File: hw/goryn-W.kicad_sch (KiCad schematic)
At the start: 19 parts, among them J1 Conn_FFC_30, U3 MT3520B, U4 MT3520B

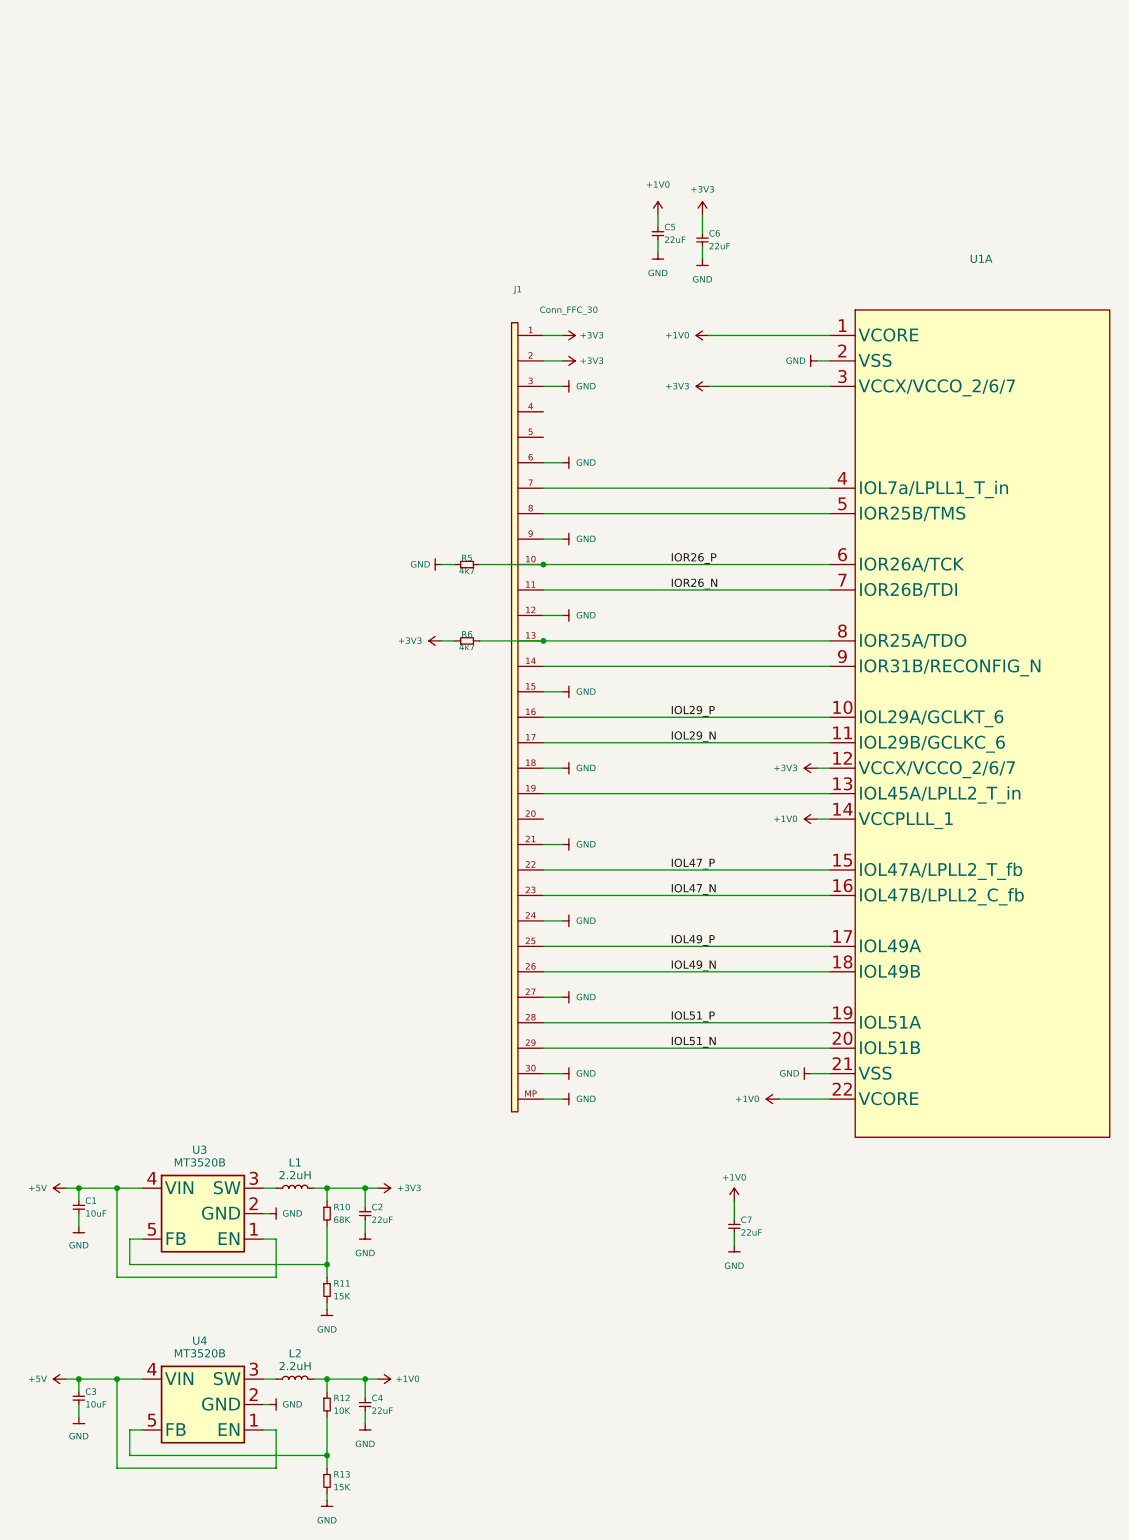
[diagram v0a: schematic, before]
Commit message: happy kicad 8
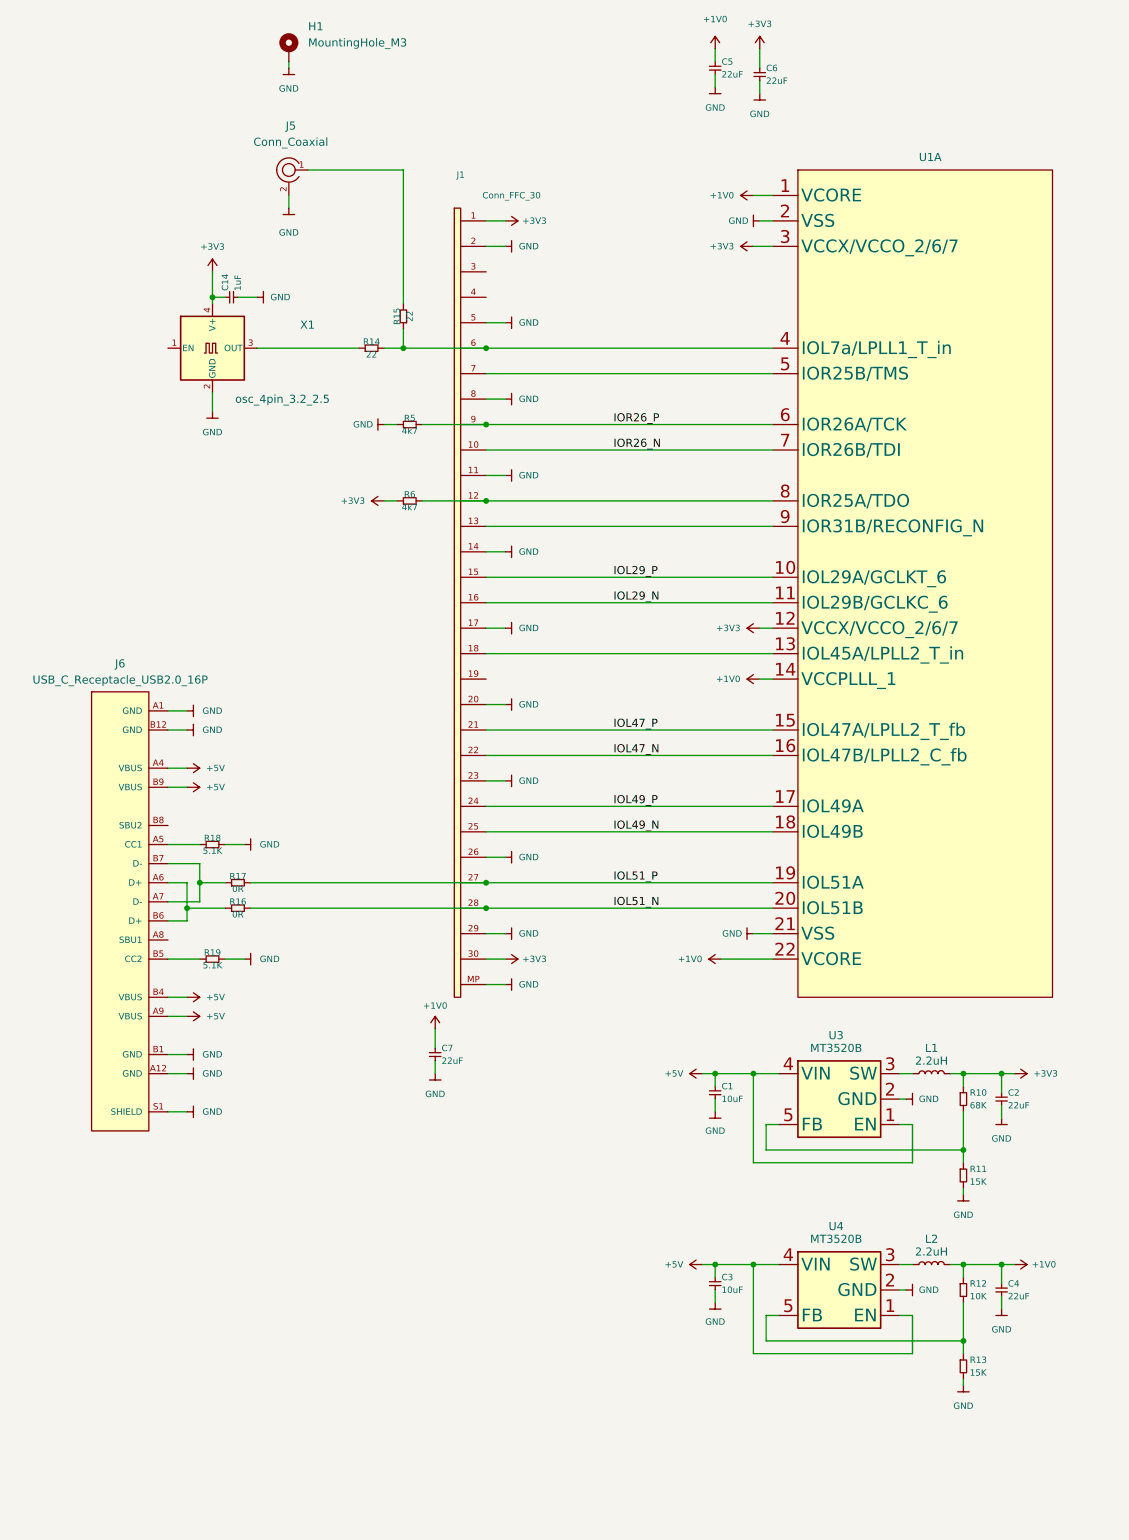
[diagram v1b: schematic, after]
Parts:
- added C14: 1uF, AI6YP:C_0603_1608Metric, symbol AI6YP:C
- added H1: MountingHole_M3, AI6YP:MountingHole_3.2mm_M3_Pad_Via, symbol AI6YP:MountingHole_M3
- added J5: Conn_Coaxial, AI6YP:U.FL_Hirose_U.FL-R-SMT-1_Vertical, symbol AI6YP:IPEX
- added J6: USB_C_Receptacle_USB2.0_16P, AI6YP:USB_C_Receptacle_GCT_USB4105-xx-A_16P_TopMnt_Horizontal, symbol AI6YP:USB_C_Receptacle_USB2.0_16P
- added R14, R15: 22, AI6YP:R_0603_1608Metric, symbol AI6YP:R
- added R16, R17: 0R, AI6YP:R_0603_1608Metric, symbol AI6YP:R
- added R18, R19: 5.1K, AI6YP:R_0603_1608Metric, symbol AI6YP:R
- added X1: osc_4pin_3.2_2.5, AI6YP:Crystal_SMD_EuroQuartz_MT-4Pin_3.2x2.5mm_HandSoldering, symbol AI6YP:osc_4pin_3.2_2.5
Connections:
- net +3V3: now also J1.30 (Pin_30), C14.1, X1.4 (V+); no longer J1.2 (Pin_2)
- net +5V: now also J6.A4 (VBUS), J6.A9 (VBUS), J6.B4 (VBUS), J6.B9 (VBUS)
- net GND: now also J1.11 (Pin_11), J1.14 (Pin_14), J1.17 (Pin_17), J1.2 (Pin_2), J1.20 (Pin_20), J1.23 (Pin_23), J1.26 (Pin_26), J1.29 (Pin_29), J1.5 (Pin_5), J1.8 (Pin_8), C14.2, H1.1, J5.2 (Ext), J6.A1 (GND), J6.A12 (GND), J6.B1 (GND), J6.B12 (GND), J6.S1 (SHIELD), R18.2, R19.2, X1.2 (GND); no longer J1.12 (Pin_12), J1.15 (Pin_15), J1.18 (Pin_18), J1.21 (Pin_21), J1.24 (Pin_24), J1.27 (Pin_27), J1.3 (Pin_3), J1.30 (Pin_30), J1.6 (Pin_6), J1.9 (Pin_9)
- net IOL29_N: now also J1.16 (Pin_16); no longer J1.17 (Pin_17)
- net IOL29_P: now also J1.15 (Pin_15); no longer J1.16 (Pin_16)
- net IOL47_N: now also J1.22 (Pin_22); no longer J1.23 (Pin_23)
- net IOL47_P: now also J1.21 (Pin_21); no longer J1.22 (Pin_22)
- net IOL49_N: now also J1.25 (Pin_25); no longer J1.26 (Pin_26)
- net IOL49_P: now also J1.24 (Pin_24); no longer J1.25 (Pin_25)
- net IOL51_N: now also J1.28 (Pin_28), R16.2; no longer J1.29 (Pin_29)
- net IOL51_P: now also J1.27 (Pin_27), R17.2; no longer J1.28 (Pin_28)
- net IOR26_N: now also J1.10 (Pin_10); no longer J1.11 (Pin_11)
- net IOR26_P: now also J1.9 (Pin_9); no longer J1.10 (Pin_10)
- net at R6.2, U1.8 (IOR25A/TDO): now also J1.12 (Pin_12); no longer J1.13 (Pin_13)
- net at U1.13 (IOL45A/LPLL2_T_in): now also J1.18 (Pin_18); no longer J1.19 (Pin_19)
- net at U1.4 (IOL7a/LPLL1_T_in): now also J1.6 (Pin_6), R14.2, R15.1; no longer J1.7 (Pin_7)
- net at U1.5 (IOR25B/TMS): now also J1.7 (Pin_7); no longer J1.8 (Pin_8)
- net at U1.9 (IOR31B/RECONFIG_N): now also J1.13 (Pin_13); no longer J1.14 (Pin_14)
- new net: J6.A7 (D-), J6.B7 (D-), R17.1
- new net: J5.1 (In), R15.2
- new net: J6.A5 (CC1), R18.1
- new net: R14.1, X1.3 (OUT)
- new net: J6.B5 (CC2), R19.1
- new net: J6.A6 (D+), J6.B6 (D+), R16.1
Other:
- moved on the sheet: C1, C2, C3, C4, C5, C6, C7, J1, L1, L2, R10, R11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

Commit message: finished routing
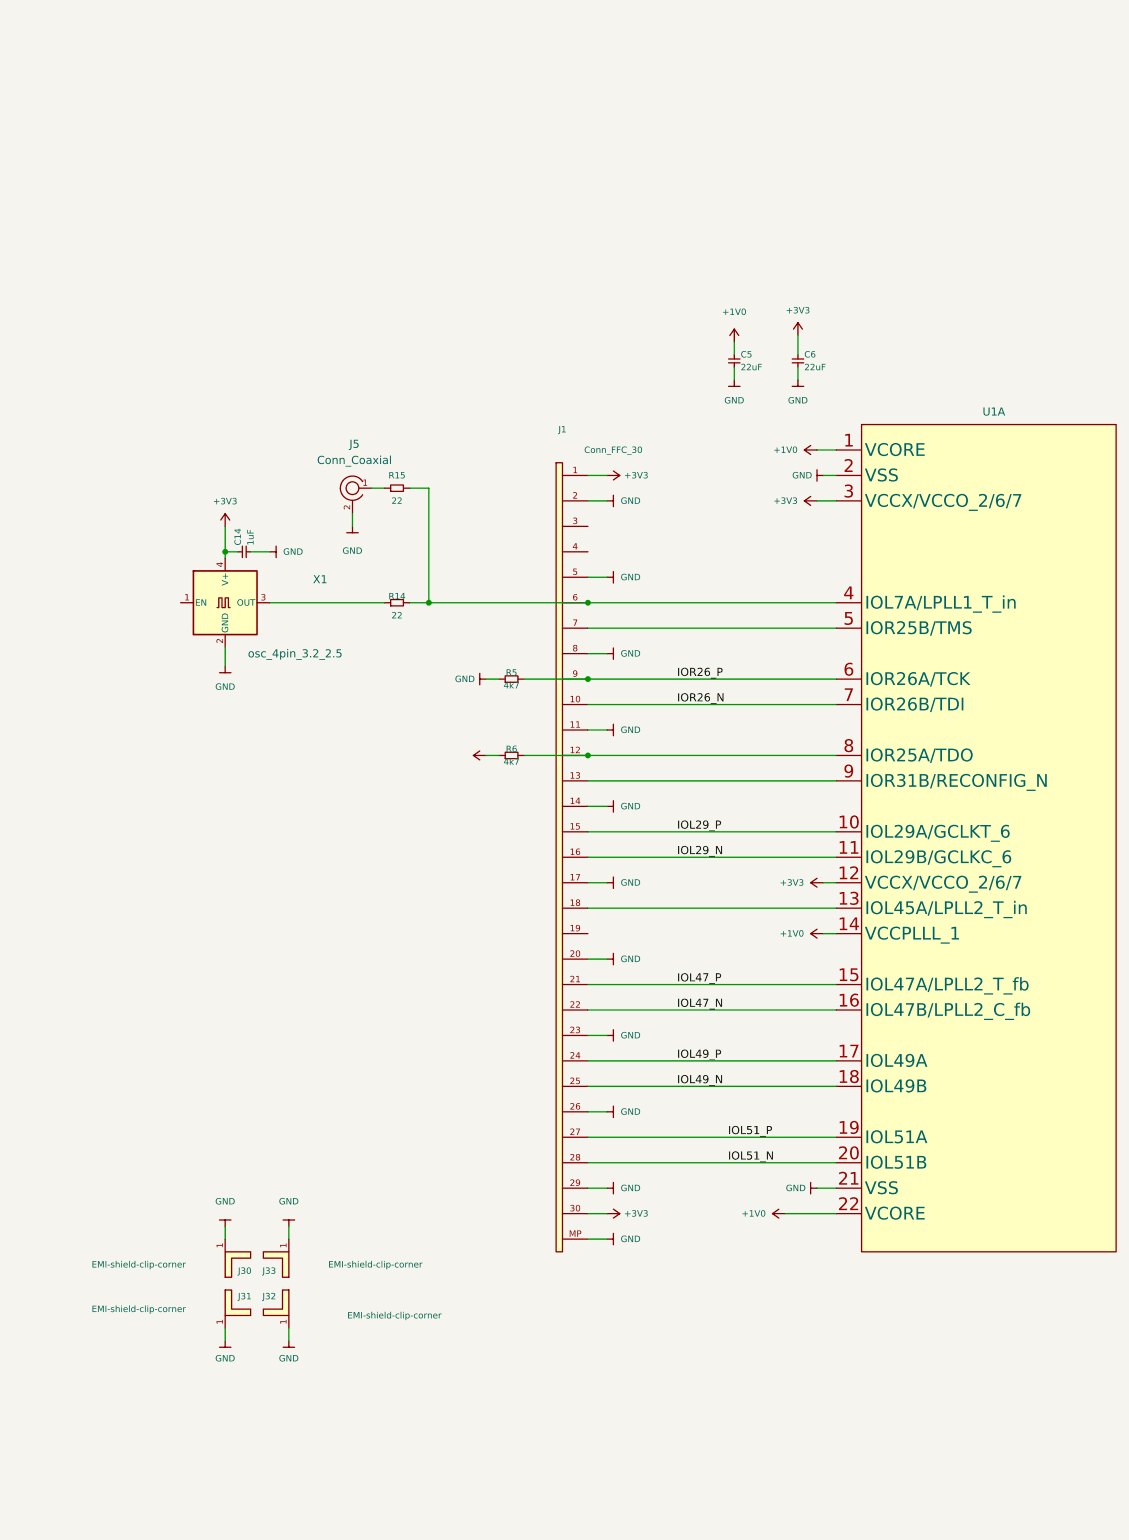
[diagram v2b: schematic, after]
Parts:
- removed C1, C3: 10uF, AI6YP:C_0603_1608Metric, symbol AI6YP:C
- removed C2, C4, C7: 22uF, AI6YP:C_0603_1608Metric, symbol AI6YP:C
- removed H1: MountingHole_M3, AI6YP:MountingHole_3.2mm_M3_Pad_Via, symbol AI6YP:MountingHole_M3
- removed J6: USB_C_Receptacle_USB2.0_16P, AI6YP:USB_C_Receptacle_GCT_USB4105-xx-A_16P_TopMnt_Horizontal, symbol AI6YP:USB_C_Receptacle_USB2.0_16P
- removed L1, L2: 2.2uH, AI6YP:L_0805_2012Metric_Pad1.05x1.20mm_HandSolder, symbol AI6YP:L
- removed R10: 68K, AI6YP:R_0603_1608Metric, symbol AI6YP:R
- removed R11, R13: 15K, AI6YP:R_0603_1608Metric, symbol AI6YP:R
- removed R12: 10K, AI6YP:R_0603_1608Metric, symbol AI6YP:R
- removed R16, R17: 0R, AI6YP:R_0603_1608Metric, symbol AI6YP:R
- removed R18, R19: 5.1K, AI6YP:R_0603_1608Metric, symbol AI6YP:R
- removed U3, U4: MT3520B, AI6YP:SOT-23-5, symbol AI6YP:MT3520B
- added J30, J31, J32, J33: EMI-shield-clip-corner, AI6YP:EMI-shield-clip-corner, symbol AI6YP:EMI-shield-clip-corner
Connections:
- net GND: now also J30.1 (Pin_1), J31.1 (Pin_1), J32.1 (Pin_1), J33.1 (Pin_1)
- net at J1.6 (Pin_6), R14.2, U1.4 (IOL7A/LPLL1_T_in): now also R15.2; no longer R15.1
- net at J5.1 (In): now also R15.1; no longer R15.2
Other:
- moved on the sheet: C14, C5, C6, J1, J5, R14, R15, R5, R6, U1A, X1

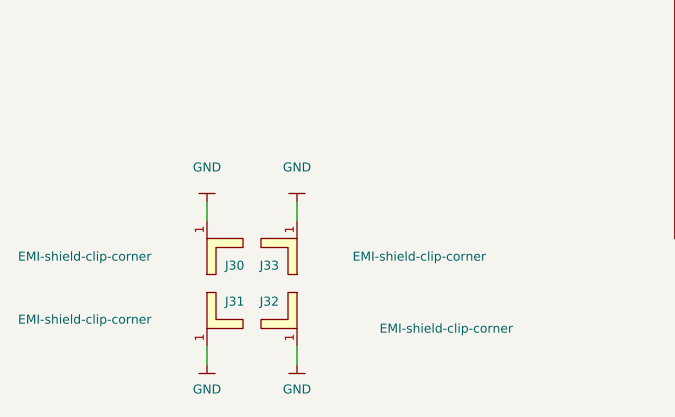
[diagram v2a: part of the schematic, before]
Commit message: v1.0.0
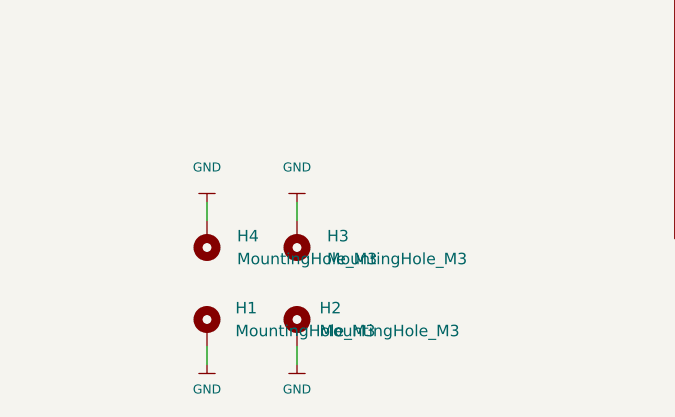
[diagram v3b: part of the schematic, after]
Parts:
- removed J30, J31, J32, J33: EMI-shield-clip-corner, AI6YP:EMI-shield-clip-corner, symbol AI6YP:EMI-shield-clip-corner
- added H1, H2, H3, H4: MountingHole_M3, AI6YP:MountingHole_3.2mm_M3_Pad_Via, symbol AI6YP:MountingHole_M3
- U1: footprint AI6YP:QFN-88-10x10mm-P0.4mm-EP6.74x6.74mm -> AI6YP:GIWIN-QFN-88-10x10mm-P0.4mm-EP6.74x6.74mm
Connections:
- net GND: now also H1.1, H2.1, H3.1, H4.1
